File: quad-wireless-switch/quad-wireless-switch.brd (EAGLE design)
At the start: 38.1 x 108 mm, 69 parts, among them IC1 LM2937IMP-3.3, Q1 DN2625K4-G, Q2 SI2323DS-T1-E3, Q3 IRL520, Q4 IRL520, Q5 IRL520, Q6 IRL520, U1 ATMEGA328P_TQFP

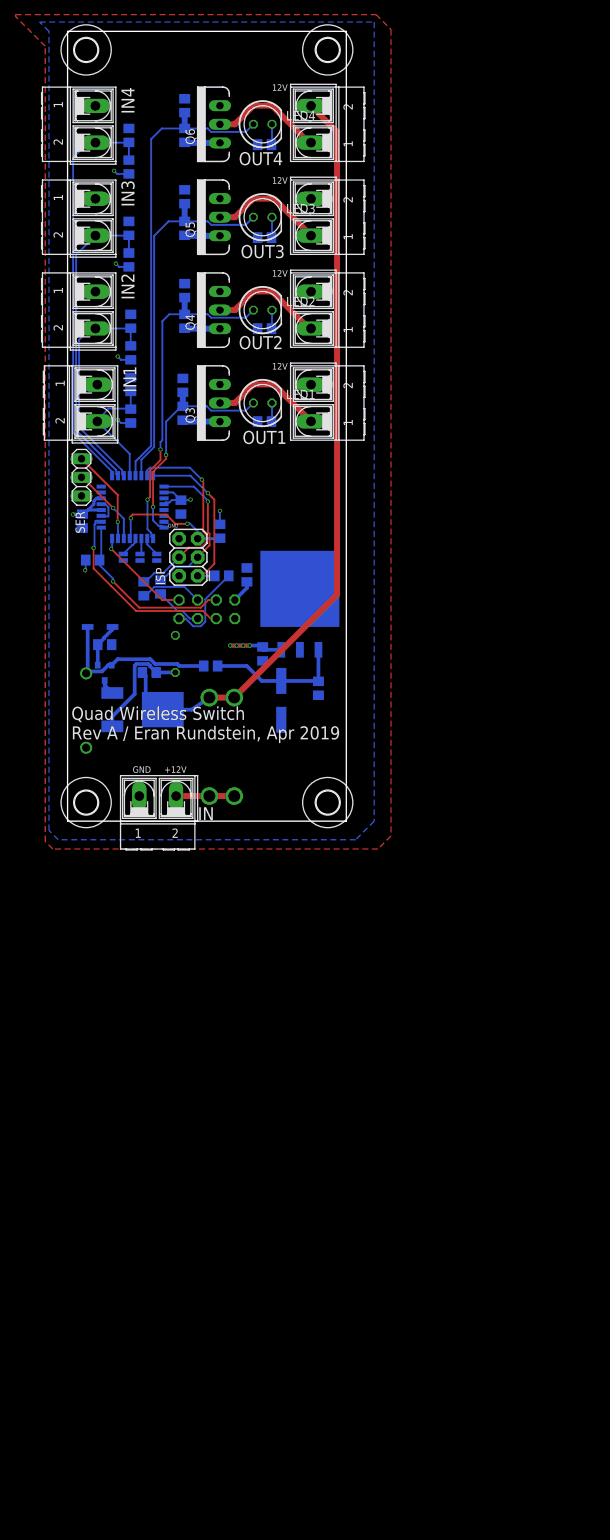
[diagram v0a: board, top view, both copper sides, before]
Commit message: quad wireless switch wip
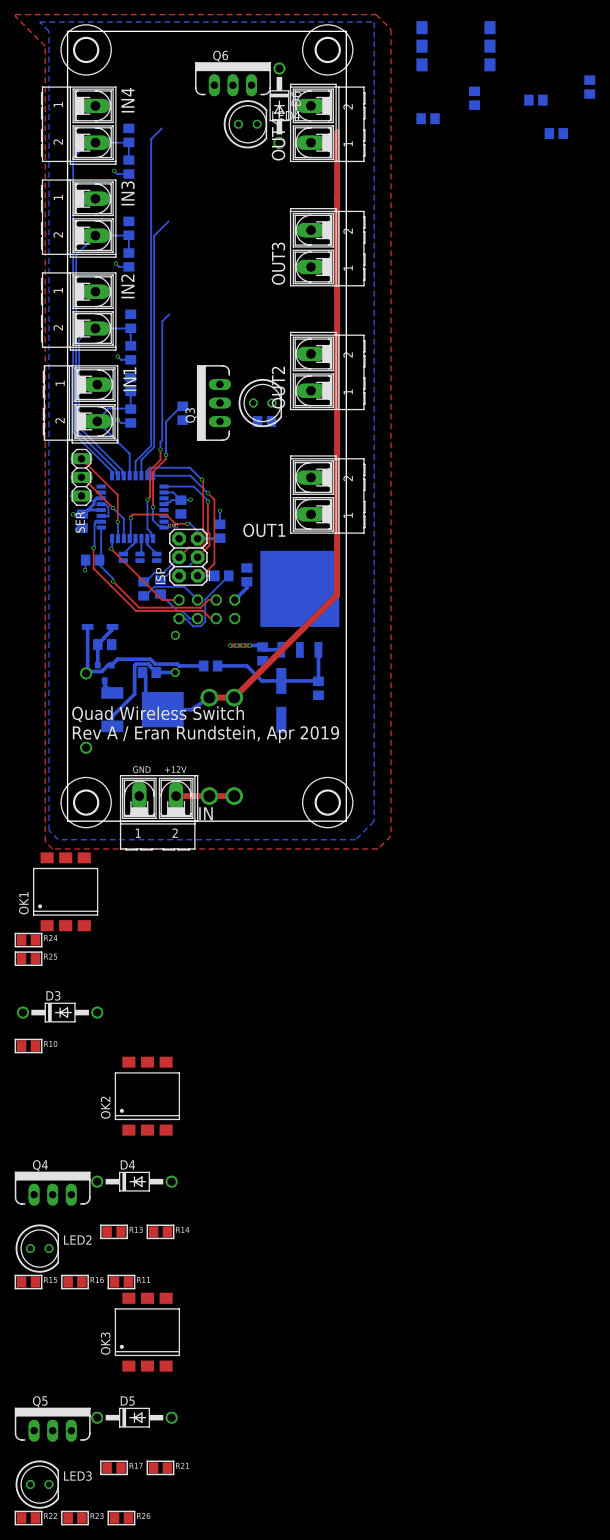
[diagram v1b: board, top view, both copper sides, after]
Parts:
- added D3, D4, D5, D6: 1N4004, diode:DO41-10
- added OK1, OK2, OK3, OK4: 4N35SM, optocoupler:DIL6-SMD
- added R24, R28, R29: 220, microbuilder:0805
- added R25, R26, R30, R31: 10K, microbuilder:0805
- added R27: 150, microbuilder:0805
- R10, R16: value 10k -> 10K
- R11: value 10k -> 150
- R13, R20, R21, R22: value 150 -> 220
- R14: value 10k -> 220
- R15, R23: value 150 -> 10K
- moved R23 189.5 mm to (1.02, -95.2), flipped to the top
- moved R17 182.4 mm to (6.35, -88.4), flipped to the top, turned to 0 degrees
- moved R22 178.0 mm to (-5.33, -95.2), flipped to the top
- moved LED3 175.9 mm to (-3.81, -90.7)
- moved Q5 167.4 mm to (-2.03, -83.3), turned to 0 degrees
- moved R16 161.5 mm to (1.02, -63.0), flipped to the top, turned to 0 degrees
- moved R21 156.4 mm to (12.7, -88.4), flipped to the top
- moved R15 145.6 mm to (-5.33, -63.0), flipped to the top, turned to 0 degrees
- moved R14 141.5 mm to (12.7, -56.1), flipped to the top, turned to 0 degrees
- moved R11 135.8 mm to (7.37, -63.0), flipped to the top, turned to 0 degrees
- moved LED2 131.8 mm to (-3.81, -58.4)
- moved R13 124.8 mm to (6.35, -56.1), flipped to the top, turned to 0 degrees
- moved Q4 123.0 mm to (-2.03, -51.1), turned to 0 degrees
- moved R10 92.7 mm to (-5.33, -30.7), flipped to the top, turned to 0 degrees
- moved OUT1 12.7 mm to (33.3, 44.5)
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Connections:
- removed net OUT2_GATE: Q4.1, R13.2
- removed net OUT3_GATE: Q5.1, R15.2
- removed net OUT4_GATE: Q6.1, R17.2
- new net N$21: OK1.5, R25.1
- new net N$23: OK1.1, R24.1
- new net N$24: D5.A, OUT3.1, Q5.2
- new net N$25: LED3.K, R21.1
- new net N$26: OK3.5, R23.1
- new net N$27: OK3.1, R22.1
- new net N$28: OK3.4, R17.1, R26.2
- new net N$29: D6.A, OUT4.1, Q6.2
- new net N$30: LED4.K, R28.1
- new net N$31: OK4.5, R30.1
- new net N$32: OK4.1, R29.1
- new net N$33: OK4.4, R27.1, R31.2
- net 12V: now also D3.C, D4.C, D5.C, D6.C, R15.2, R23.2, R25.2, R30.2
- net GND: now also OK1.2, OK2.2, OK3.2, OK4.2, R10.1, R13.2, R16.1, R26.1, R28.2, R31.1; no longer R10.2, R11.2, R14.2, R16.2, R22.2, R23.2
- net N$18: now also OK2.1, R14.1; no longer OUT3.1, Q5.2
- net N$2: now also OK1.4, R10.2, R12.1; no longer LED2.K, R21.1
- net N$22: now also OK2.4, R11.1, R16.2; no longer OUT4.1, Q6.2
- net N$3: now also D4.A, OUT2.1, Q4.2; no longer LED3.K, R22.1
- net N$4: now also LED2.K, R13.1; no longer LED4.K, R23.1
- net N$6: now also D3.A
- net N$8: now also OK2.5, R15.1; no longer OUT2.1, Q4.2
- net OUT1: now also R24.2; no longer R10.1, R12.1
- net OUT1_GATE: now also Q4.1, Q5.1, Q6.1, R11.2, R17.2, R27.2
- net OUT2: now also R14.2; no longer R11.1, R13.1
- net OUT3: now also R22.2; no longer R14.1, R15.1
- net OUT4: now also R29.2; no longer R16.1, R17.1
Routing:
- net 12V: track 116.8 -> 101.1 mm
- net N$22: track 15.6 -> 0.00 mm
- net N$18: track 15.6 -> 0.00 mm
- net N$8: track 15.6 -> 0.00 mm
- net N$6: track 15.6 -> 0.00 mm
- net OUT4: track 64.2 -> 48.9 mm
- net OUT3: track 50.9 -> 36.3 mm
- net OUT2: track 46.6 -> 32.2 mm
- net OUT1: track 31.5 -> 19.1 mm
- net OUT1_GATE: track 5.16 -> 0.27 mm
- net OUT4_GATE: track 4.85 -> 0.00 mm
- net OUT2_GATE: track 4.85 -> 0.00 mm
- net OUT3_GATE: track 4.85 -> 0.00 mm
- net N$4: track 2.82 -> 0.00 mm
- net N$3: track 2.82 -> 0.00 mm
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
